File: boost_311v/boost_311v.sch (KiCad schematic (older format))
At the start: 58 parts, among them J1 Vin_Cnt, J2 VO, J3 Vin_boost, Q1 BC556, Q2 PN2222A, Q5 IRFP260, U1 LM358, U2 L7812, U3 TC4420CPA, U4 LF357, U5 NE555

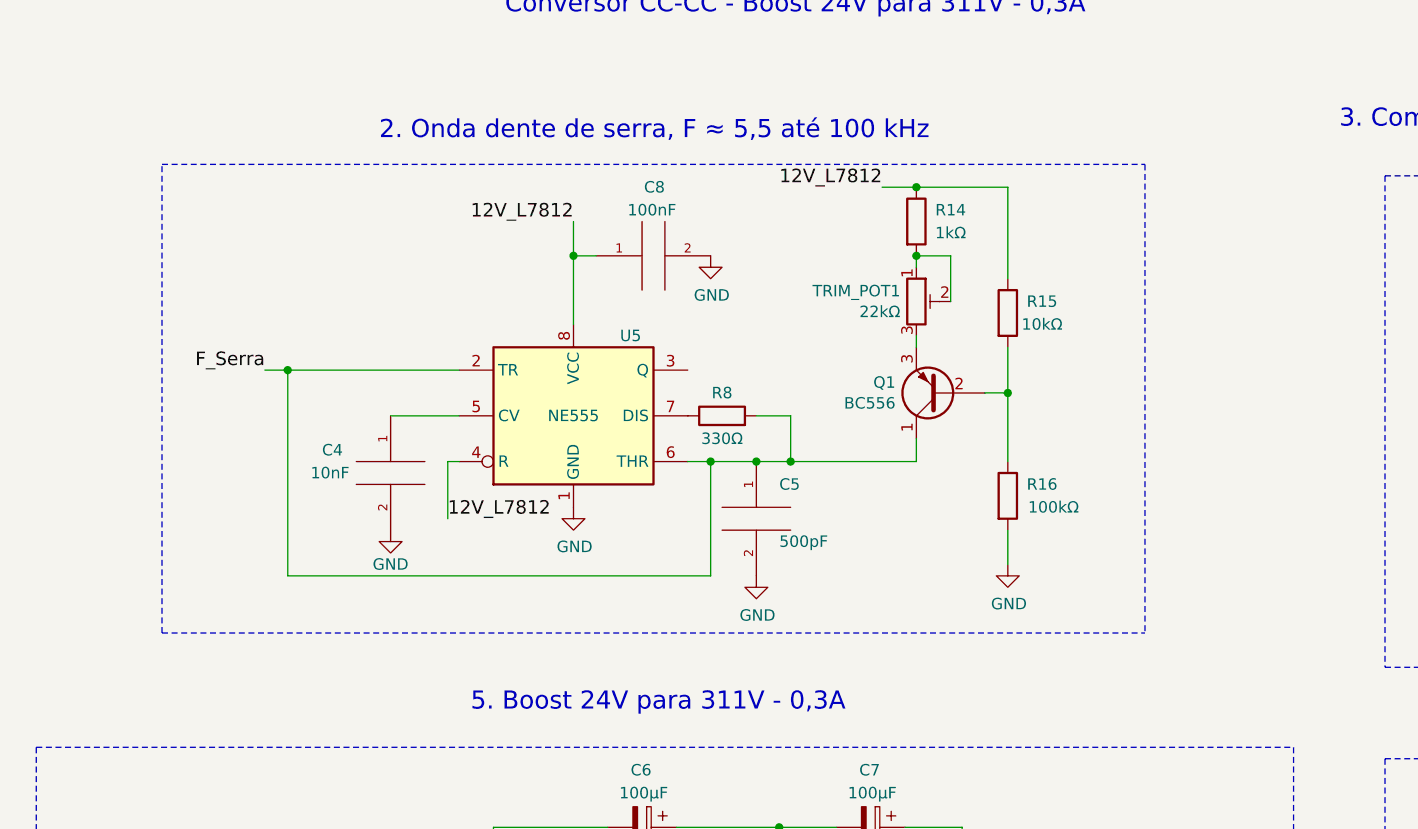
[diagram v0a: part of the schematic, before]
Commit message: Up ocb
Signed-off-by: fgl27 <fglfgl27@gmail.com>
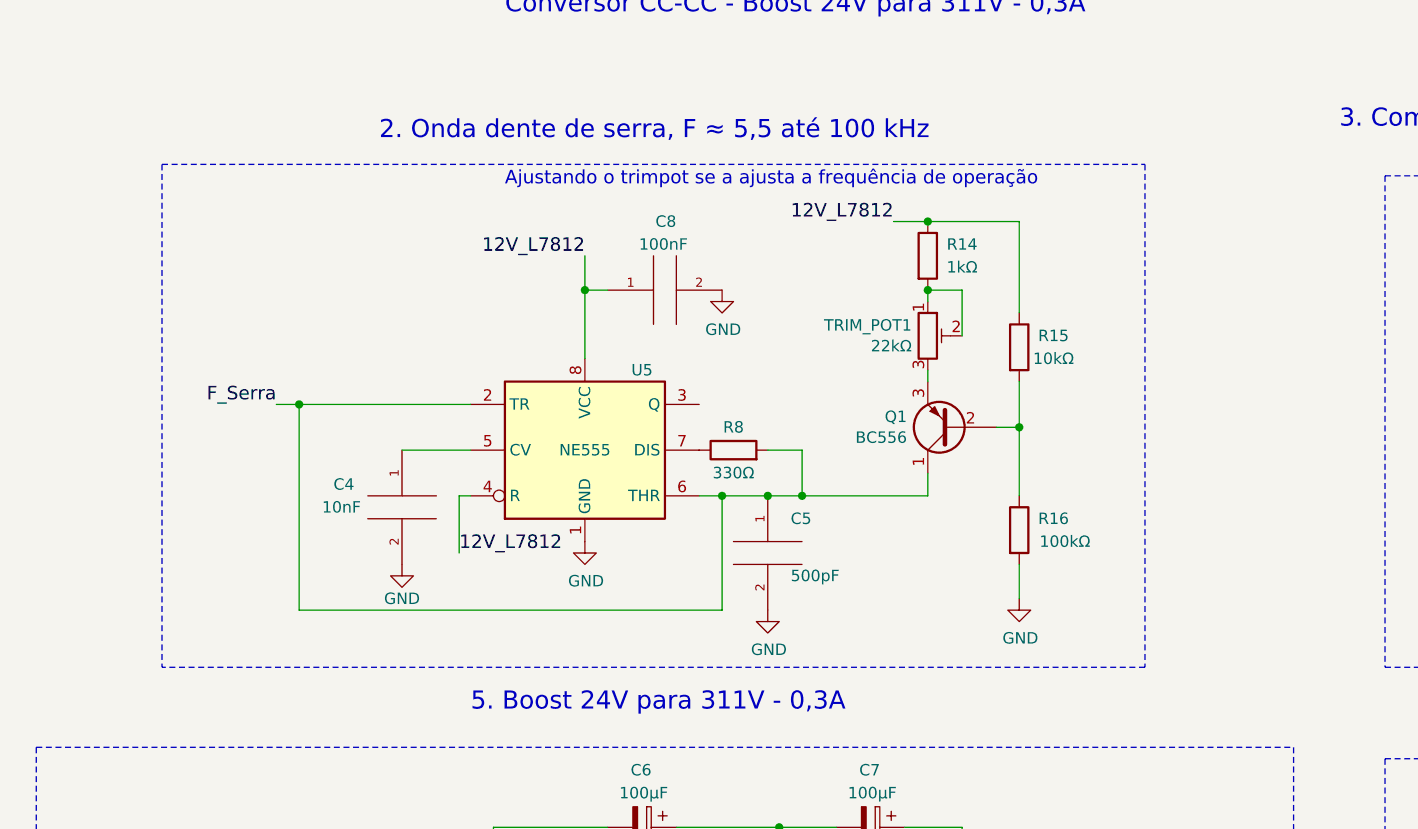
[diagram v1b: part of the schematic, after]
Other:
- note added: "Ajustando o trimpot se a ajusta a frequência de operação"
- moved on the sheet: C4, C5, C8, Q1, R14, R15, R16, R8, TRIM_POT1, U5

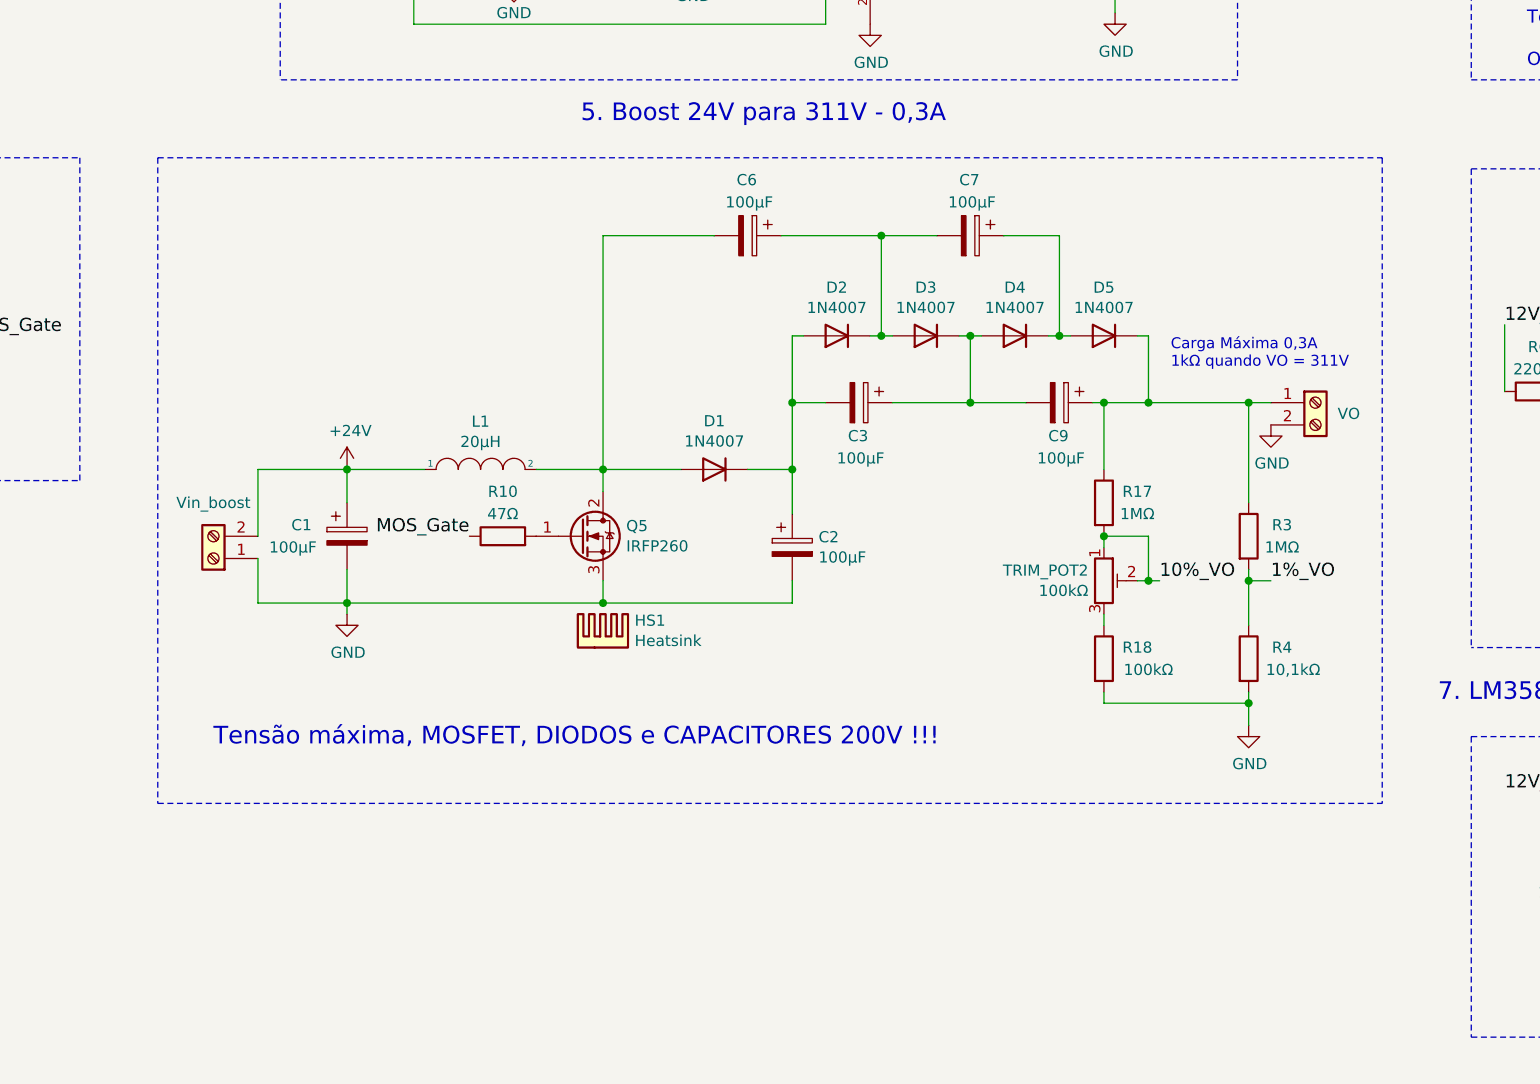
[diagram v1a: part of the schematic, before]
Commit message: Up pcb
Signed-off-by: fgl27 <fglfgl27@gmail.com>
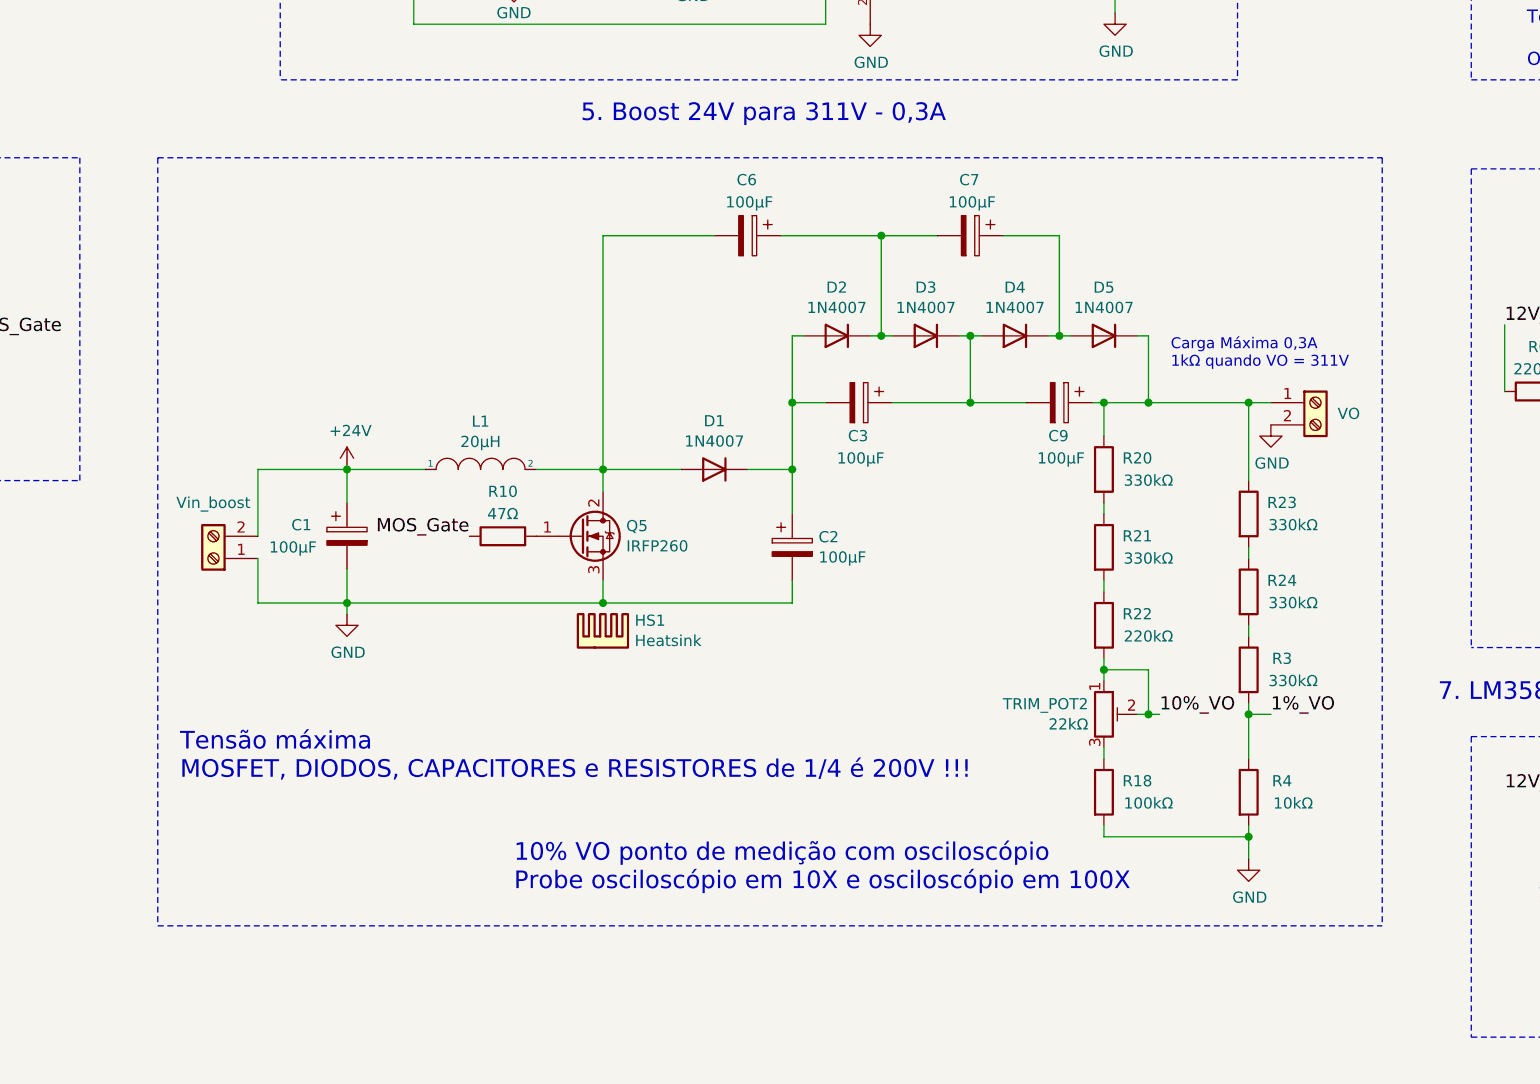
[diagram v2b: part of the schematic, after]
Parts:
- removed R17: 1MΩ, Resistor_THT:R_Axial_DIN0207_L6.3mm_D2.5mm_P10.16mm_Horizontal, symbol Device:R
- added R20, R21, R23, R24: 330kΩ, Resistor_THT:R_Axial_DIN0207_L6.3mm_D2.5mm_P10.16mm_Horizontal, symbol Device:R
- added R22: 220kΩ, Resistor_THT:R_Axial_DIN0207_L6.3mm_D2.5mm_P10.16mm_Horizontal, symbol Device:R
- R3: value 1MΩ -> 330kΩ
- R4: value 10,1kΩ -> 10kΩ
- TRIM_POT2: value 100kΩ -> 22kΩ
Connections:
- net 10%_VO: now also R22.2
- net at C9.1, D5.1 (K), J2.1 (Pin_1): now also R20.1, R23.1; no longer R3.1
- new net: R23.2, R24.1
- new net: R24.2, R3.1
- new net: R21.2, R22.1
- new net: R20.2, R21.1
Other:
- note added: "10% VO ponto de medição com osciloscópio\nProbe osciloscópio em 10X e osciloscópio em 100X"
- note added: "Tensão máxima\nMOSFET, DIODOS, CAPACITORES e RESISTORES de 1/4 é 200V !!!"
- note removed: "Tensão máxima, MOSFET, DIODOS e CAPACITORES 200V !!!"
- moved on the sheet: R18, R3, R4, TRIM_POT2
